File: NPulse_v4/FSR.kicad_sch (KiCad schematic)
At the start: 15 parts, among them J10 Conn_02x05_Odd_Even, J5 Conn_02x05_Odd_Even, U11 TLV70233_WSON6

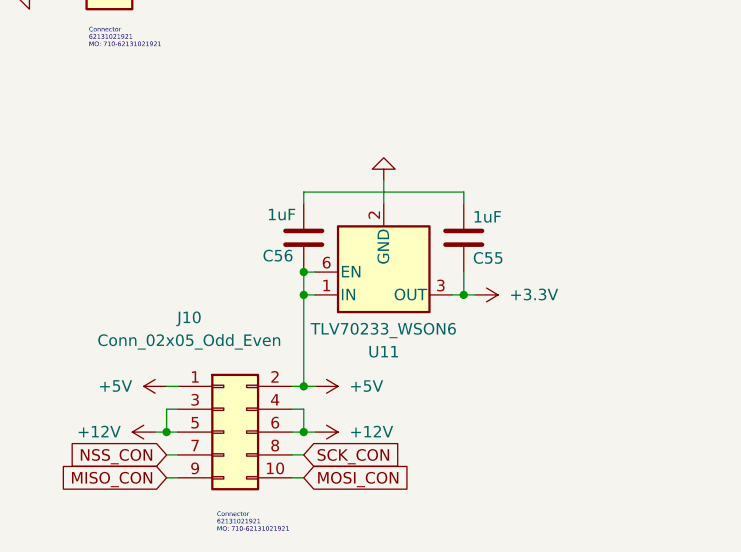
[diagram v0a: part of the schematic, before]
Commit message: some modifications on the routing
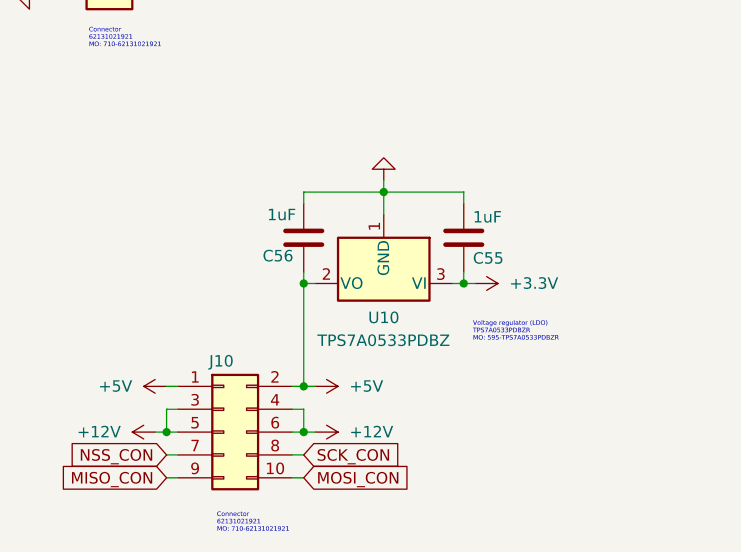
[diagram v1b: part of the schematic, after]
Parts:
- removed U11: TLV70233_WSON6, Package_SON:Texas_X2SON-4_1x1mm_P0.65mm, symbol Regulator_Linear:TLV70233_WSON6
- added U10: TPS7A0533PDBZ, Package_TO_SOT_SMD:SOT-23, symbol Regulator_Linear:TPS7A0533PDBZ
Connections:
- net +3.3V: now also U10.3 (VI)
- net +5V: now also U10.2 (VO)
- net GND: now also C55.2, C56.2, U10.1 (GND)
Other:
- note added: "Voltage regulator (LDO) TPS7A0533PDBZR MO: 595-TPS7A0533PDBZR"
